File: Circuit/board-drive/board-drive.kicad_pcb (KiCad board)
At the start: 2 copper layers, 164.4 x 98.3 mm, 32 parts, among them M3 MountingHole_3.2mm_M3, P1 XT30, P10 XT60, P2 XT30, P3 XT30, P4 XT30, P5 XT30, P6 XT30, P7 XT30, P8 XT30, P9 XT60, U1 Pololu_Maestro12, U10 PowerDist_WiretoBoard, U11 PowerDist_WiretoBoard, U16 PowerDist_WiretoBoard, U17 PowerDist_WiretoBoard, U18 PowerDist_WiretoBoard, U19 PowerDist_WiretoBoard, U2 Si8660BA-B-IS1, U3 Si8660BA-B-IS1, U8 PowerDist_WiretoBoard, U9 PowerDist_WiretoBoard

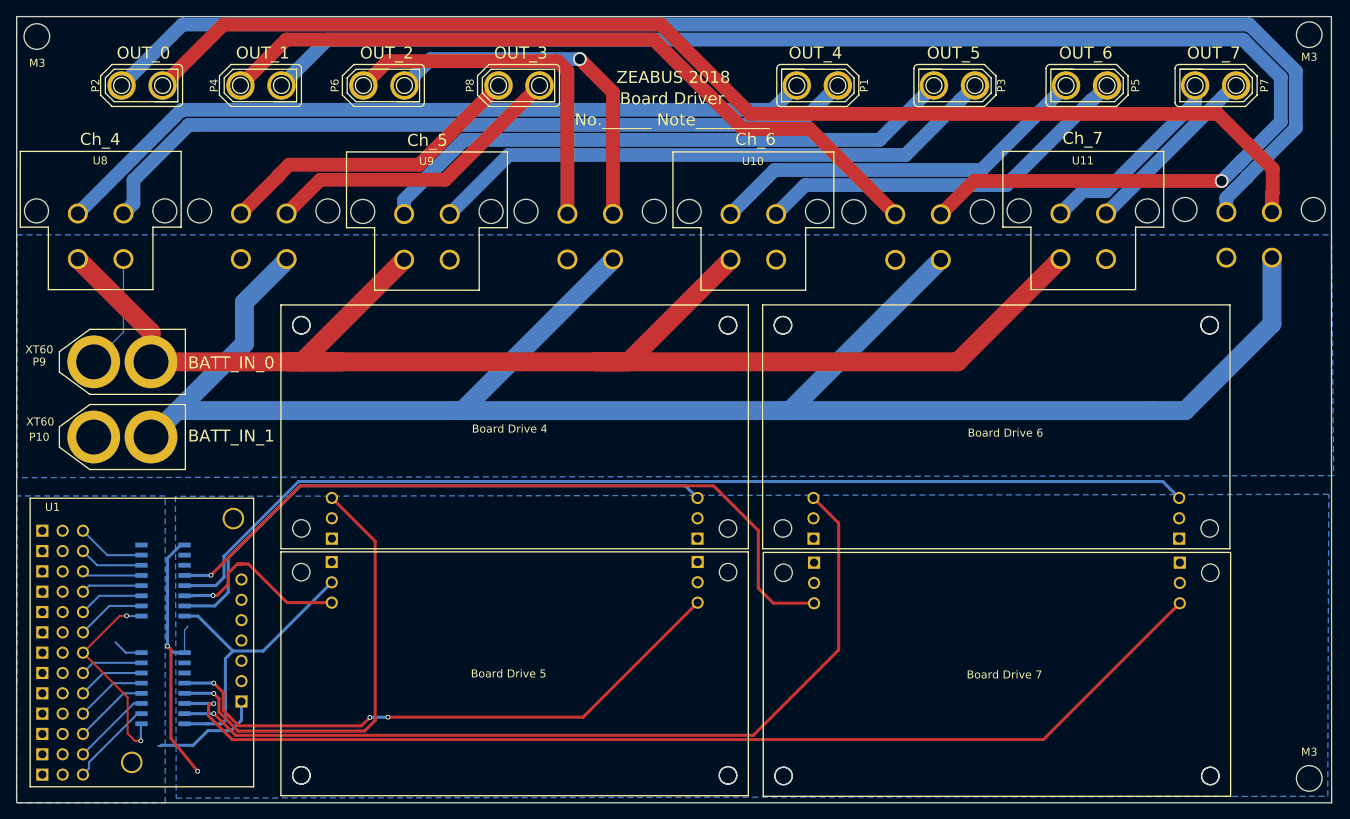
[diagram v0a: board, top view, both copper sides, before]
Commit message: edited pcb
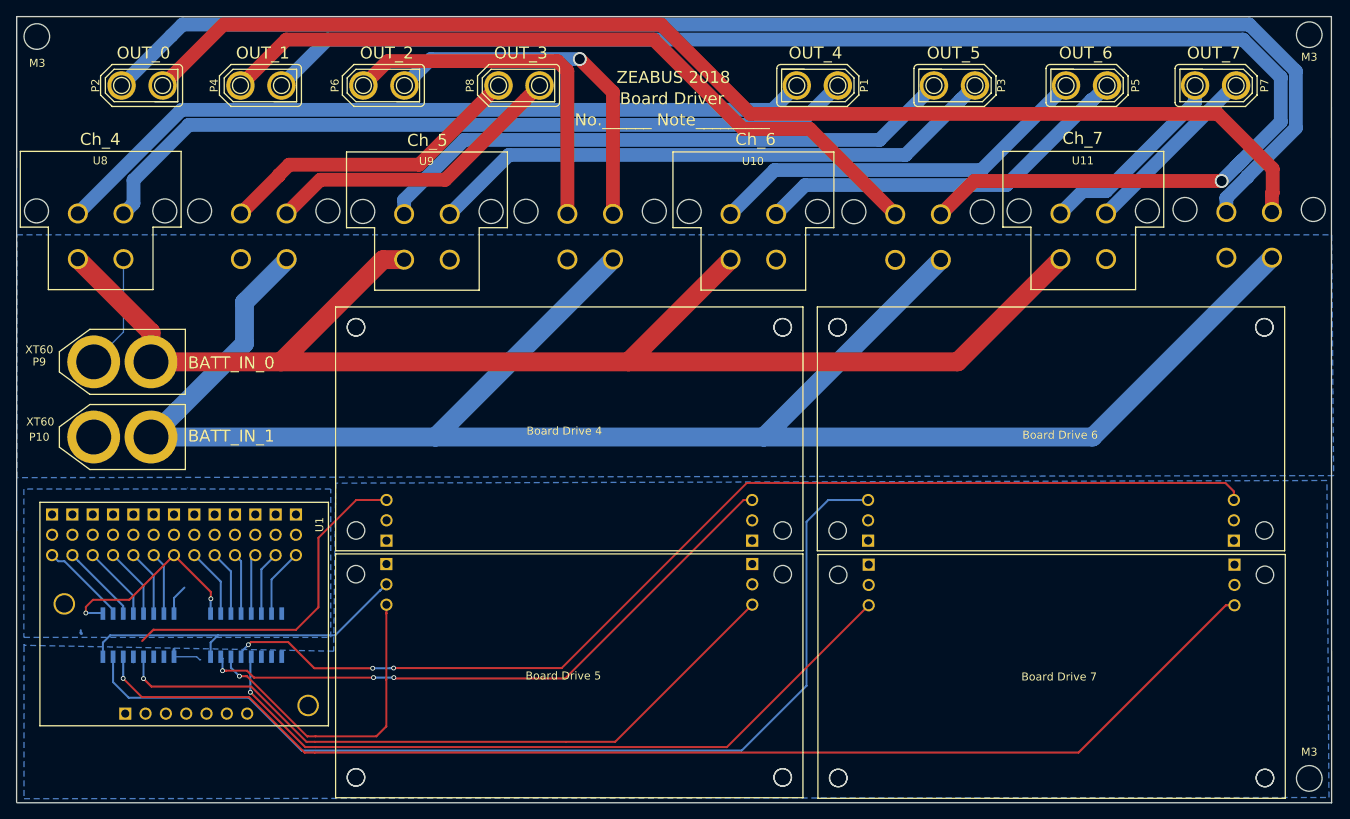
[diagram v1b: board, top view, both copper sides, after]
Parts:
- moved U1 27.8 mm to (52.9, 140.5), turned to 90 degrees
- moved U3 12.4 mm to (78.7, 129.2), turned to 0 degrees
- moved U2 7.31 mm to (65.2, 129.2), turned to 0 degrees
- moved Board Drive 0 6.84 mm to (150.1, 118.6)
- moved Board Drive 1 6.84 mm to (208.6, 119.1)
- moved Board Drive 6 6.84 mm to (208.5, 118.6)
- moved Board Drive 7 6.84 mm to (150.2, 119.1)
- moved Board Drive 2 6.84 mm to (89.9, 118.6)
- moved Board Drive 5 6.84 mm to (89.9, 119.0)
- moved Board Drive 3 6.84 mm to (148.3, 119.0)
- moved Board Drive 4 6.84 mm to (148.3, 118.6)
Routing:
- net GNDA: track 37.7 -> 4.89 mm, vias 2 -> 0
- net /signal0: track 108.7 -> 127.2 mm, vias 1 -> 0
- net /signal1: track 136.2 -> 153.9 mm
- net /signal7: track 24.2 -> 41.6 mm
- net /signal3: track 75.3 -> 90.5 mm, vias 3 -> 1
- net /signal2: track 58.5 -> 44.0 mm, vias 1 -> 0
- net GNDD: track 17.9 -> 4.23 mm
- net /BATTIN_0: track 182.7 -> 174.4 mm
- net /BATTIN_1: track 234.3 -> 241.3 mm
- net /signal8: track 132.6 -> 138.2 mm, vias 0 -> 3
- net /+5v_BEC: track 38.3 -> 43.7 mm
- net /signal6: track 73.5 -> 77.7 mm, vias 0 -> 3
- net /signal9: track 93.8 -> 92.1 mm
